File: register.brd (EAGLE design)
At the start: 100 x 80 mm, 28 parts, among them IC1 74AS574N, IC2 74AS574N, IC3 74AC283N, IC4 74AC283N, IC5 74AC283N, IC6 74AC283N, IC7 74AC244N, IC8 74AC244N

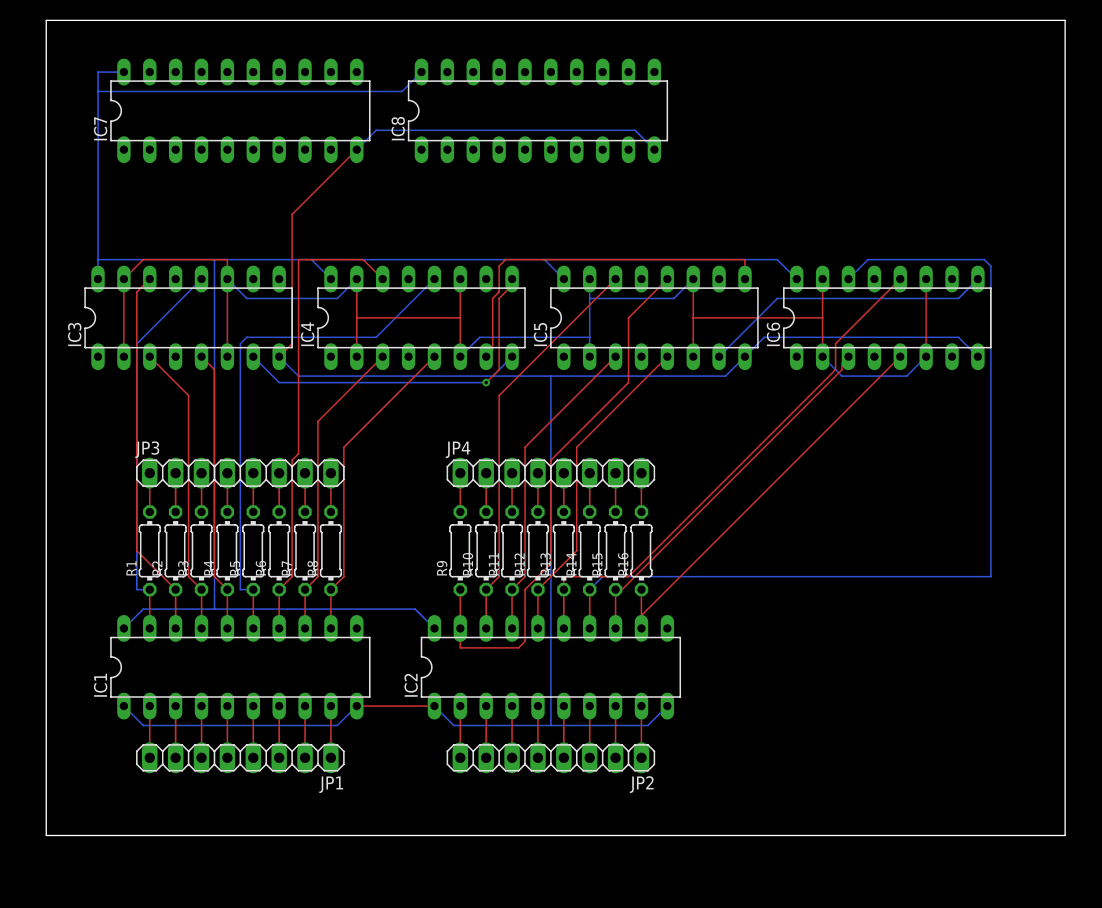
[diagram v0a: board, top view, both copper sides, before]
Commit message: some work
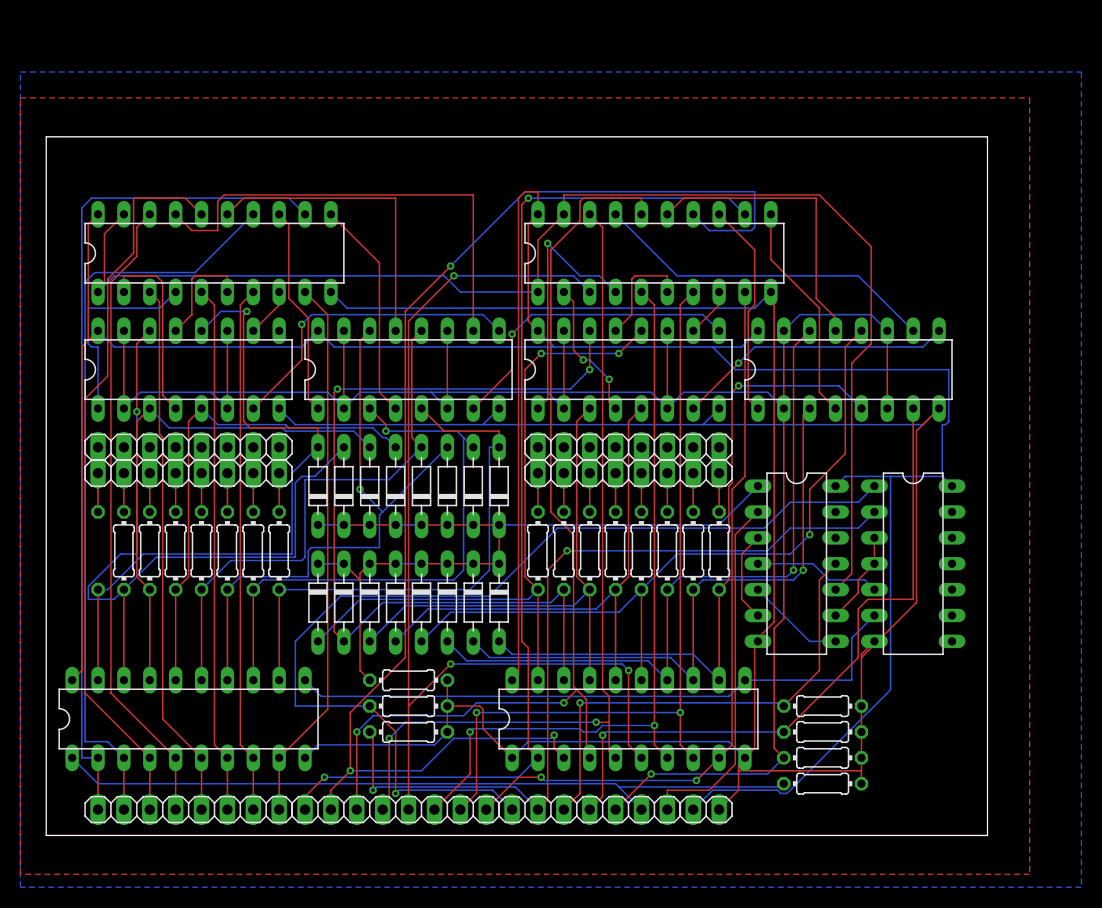
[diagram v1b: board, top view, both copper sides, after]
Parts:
- added D1, D10, D11, D12, D13, D14, D15, D16, D2, D3, D4, D5, D6, D7, D8, D9: (no value), diode:D-7.5
- added IC10: AND(08), 74xx-us:DIL14
- added IC9: NOT(04), 74xx-us:DIL14
- added JP5: (no value), pinhead:1X07
- added JP6, JP7: (no value), pinhead:1X08
- added JP8: (no value), pinhead:1X02
- added R17, R18, R19, R20, R21, R22, R23: 10k, rcl:0204/7
- IC1, IC2: value 74AS574N -> D(574)
- IC3, IC4, IC5, IC6: value 74AC283N -> ADD(283)
- IC7, IC8: value 74AC244N -> BUF(244)
- moved IC8 18.1 mm to (59.7, 57.1)
- moved JP2 16.1 mm to (34.3, 2.54)
- moved IC7 14.2 mm to (16.5, 57.1)
- moved IC2 9.16 mm to (57.1, 11.4)
- moved R11 7.62 mm to (53.3, 27.9)
- moved R12 7.62 mm to (55.9, 27.9)
- moved R13 7.62 mm to (58.4, 27.9)
- moved R16 7.62 mm to (66.0, 27.9)
- moved JP4 7.62 mm to (57.1, 35.6)
- moved R10 7.62 mm to (50.8, 27.9)
- moved R14 7.62 mm to (61.0, 27.9)
- moved R15 7.62 mm to (63.5, 27.9)
- moved R9 7.62 mm to (48.3, 27.9)
- moved IC1 7.18 mm to (14.0, 11.4)
- moved JP1 7.18 mm to (14.0, 2.54)
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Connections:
- removed net LSB: IC2.9, JP2.1
- removed net MSB: IC1.2, JP1.8
- removed net N$10: IC1.8, JP1.2
- removed net N$11: IC1.7, JP1.3
- removed net N$12: IC1.6, JP1.4
- removed net N$13: IC1.5, JP1.5
- removed net N$14: IC1.4, JP1.6
- removed net N$15: IC1.3, JP1.7
- removed net N$8: IC2.2, JP2.8
- removed net N$9: IC1.9, JP1.1
- new net 8BIT: IC1.1, JP5.2, R23.1
- new net B0: IC2.9, IC8.9, JP2.1
- new net B1: IC2.8, IC8.7, JP2.2
- new net B10: IC1.7, IC7.5, JP1.3
- new net B11: IC1.6, IC7.3, JP1.4
- new net B12: IC1.5, IC7.18, JP1.5
- new net B13: IC1.4, IC7.16, JP1.6
- new net B14: IC1.3, IC7.14, JP1.7
- new net B15: IC1.2, IC7.12, JP1.8
- new net B2: IC2.7, IC8.5, JP2.3
- new net B3: IC2.6, IC8.3, JP2.4
- new net B4: IC2.5, IC8.18, JP2.5
- new net B5: IC2.4, IC8.16, JP2.6
- new net B6: IC2.3, IC8.14, JP2.7
- new net B7: IC2.2, IC8.12, JP2.8
- new net B8: IC1.9, IC7.9, JP1.1
- new net B9: IC1.8, IC7.7, JP1.2
- new net CLK: IC10.1, JP5.7, R18.1
- new net CLK2: IC1.11, IC10.6, IC2.11
- new net N$18: IC3.4, IC7.2
- new net N$19: IC3.1, IC7.4
- new net N$20: IC3.13, IC7.6
- new net N$21: IC3.10, IC7.8
- new net N$22: IC4.4, IC7.11
- new net N$23: IC4.1, IC7.13
- new net N$24: IC4.13, IC7.15
- new net N$25: IC4.10, IC7.17
- new net N$26: IC5.4, IC8.2
- new net N$27: IC5.1, IC8.4
- new net N$28: IC5.13, IC8.6
- new net N$29: IC5.10, IC8.8
- new net N$30: IC6.4, IC8.11
- new net N$47: IC6.1, IC8.13
- new net N$48: IC6.13, IC8.15
- new net N$49: IC6.10, IC8.17
- new net RD: IC9.11, JP5.5, R20.1
- new net WE: IC10.2, JP5.6, R19.1
- new net Z: IC9.2, JP5.1
- net DEC: now also JP5.3, R22.1
- net GND: now also IC10.7, IC9.7, JP8.1, R17.1, R18.2, R19.2, R20.2, R21.2, R22.2, R23.2; no longer IC1.1
- net INC: now also JP5.4, R21.1
- net N$2: now also IC10.3, IC10.4, IC9.9; no longer IC2.8, JP2.2
- net N$3: now also D1.C, D10.C, D11.C, D12.C, D13.C, D14.C, D15.C, D16.C, D2.C, D3.C, D4.C, D5.C, D6.C, D7.C, D8.C, D9.C, IC9.1, R17.2; no longer IC2.7, JP2.3
- net N$31: now also JP7.1
- net N$32: now also JP7.2
- net N$33: now also JP7.3
- net N$34: now also JP7.4
- net N$35: now also JP7.5
- net N$36: now also JP7.6
- net N$37: now also JP7.7
- net N$38: now also JP7.8
- net N$39: now also JP6.1
- net N$4: now also IC7.1, IC7.19, IC8.1, IC8.19, IC9.10; no longer IC2.6, JP2.4
- net N$40: now also JP6.2
- net N$41: now also JP6.3
- net N$42: now also JP6.4
- net N$43: now also JP6.5
- net N$44: now also JP6.6
- net N$45: now also JP6.7
- net N$46: now also JP6.8
- net N$5: now also IC10.5, IC9.4; no longer IC2.5, JP2.5
- net N$6: now also IC9.3, IC9.6; no longer IC2.4, JP2.6
- net N$7: now also IC9.5, IC9.8; no longer IC2.3, JP2.7
- net Q0: now also D16.A
- net Q1: now also D15.A
- net Q10: now also D6.A
- net Q11: now also D5.A
- net Q12: now also D4.A
- net Q13: now also D3.A
- net Q14: now also D2.A
- net Q15: now also D1.A
- net Q2: now also D14.A
- net Q3: now also D13.A
- net Q4: now also D12.A
- net Q5: now also D11.A
- net Q6: now also D10.A
- net Q7: now also D9.A
- net Q8: now also D8.A
- net Q9: now also D7.A
- net VCC: now also IC10.14, IC9.14, JP8.2
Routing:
- net N$4: track 5.08 -> 131.1 mm
- net B6: track 0.00 -> 125.5 mm, vias 0 -> 3
- net B7: track 0.00 -> 103.5 mm, vias 0 -> 2
- net B3: track 0.00 -> 100.9 mm, vias 0 -> 3
- net CLK: track 0.00 -> 98.8 mm, vias 0 -> 1
- net B5: track 0.00 -> 96.0 mm, vias 0 -> 2
- net B4: track 0.00 -> 83.9 mm, vias 0 -> 2
- net B15: track 0.00 -> 83.6 mm
- net WE: track 0.00 -> 81.4 mm, vias 0 -> 2
- net VCC: track 196.5 -> 274.6 mm
- net B1: track 0.00 -> 77.0 mm, vias 0 -> 2
- net B2: track 0.00 -> 74.5 mm, vias 0 -> 2
- net 8BIT: track 0.00 -> 74.3 mm
- net B14: track 0.00 -> 73.9 mm
- net N$3: track 5.08 -> 78.3 mm
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- added copper zone on layer 1, net GND
- added copper zone on layer 16, net GND
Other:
- board size 100 x 80 mm -> 92.4 x 68.6 mm
